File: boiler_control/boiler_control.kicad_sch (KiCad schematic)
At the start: 21 parts, among them J1 Conn_01x01, J3V3 Conn_01x03, J5V1 Conn_01x03, U2 MOUDLE-SEEEDUINO-XIAO-ESP32C3

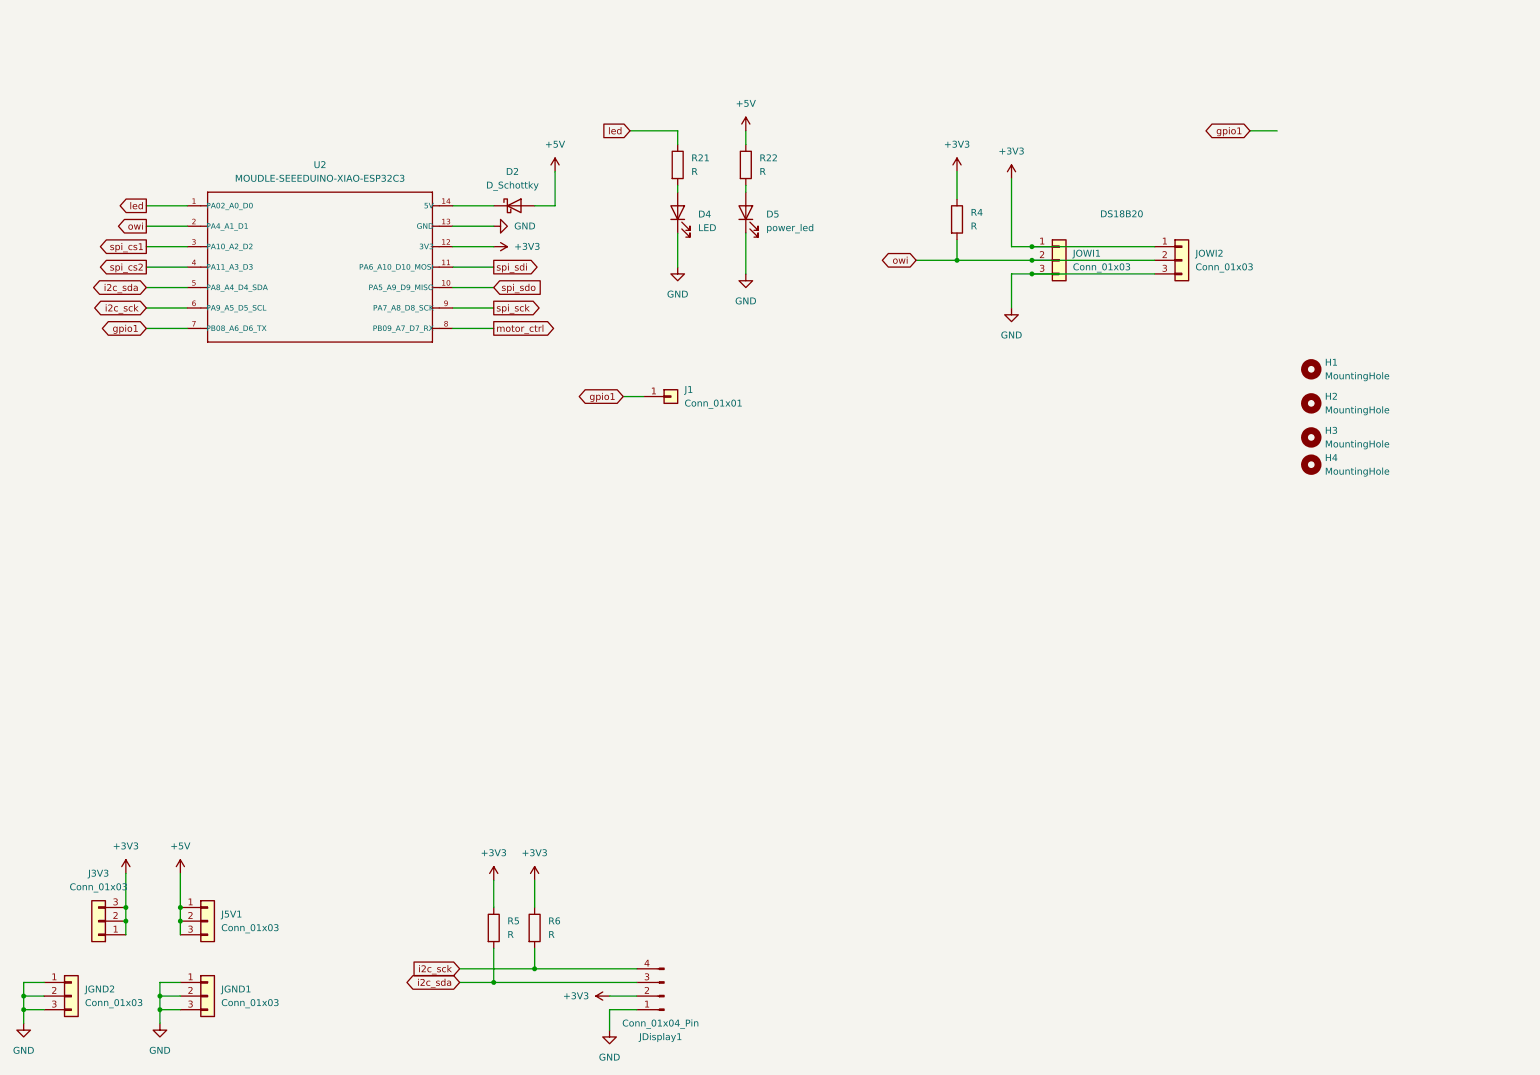
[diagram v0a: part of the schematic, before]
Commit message: Updating to v1.4 - pushed to order
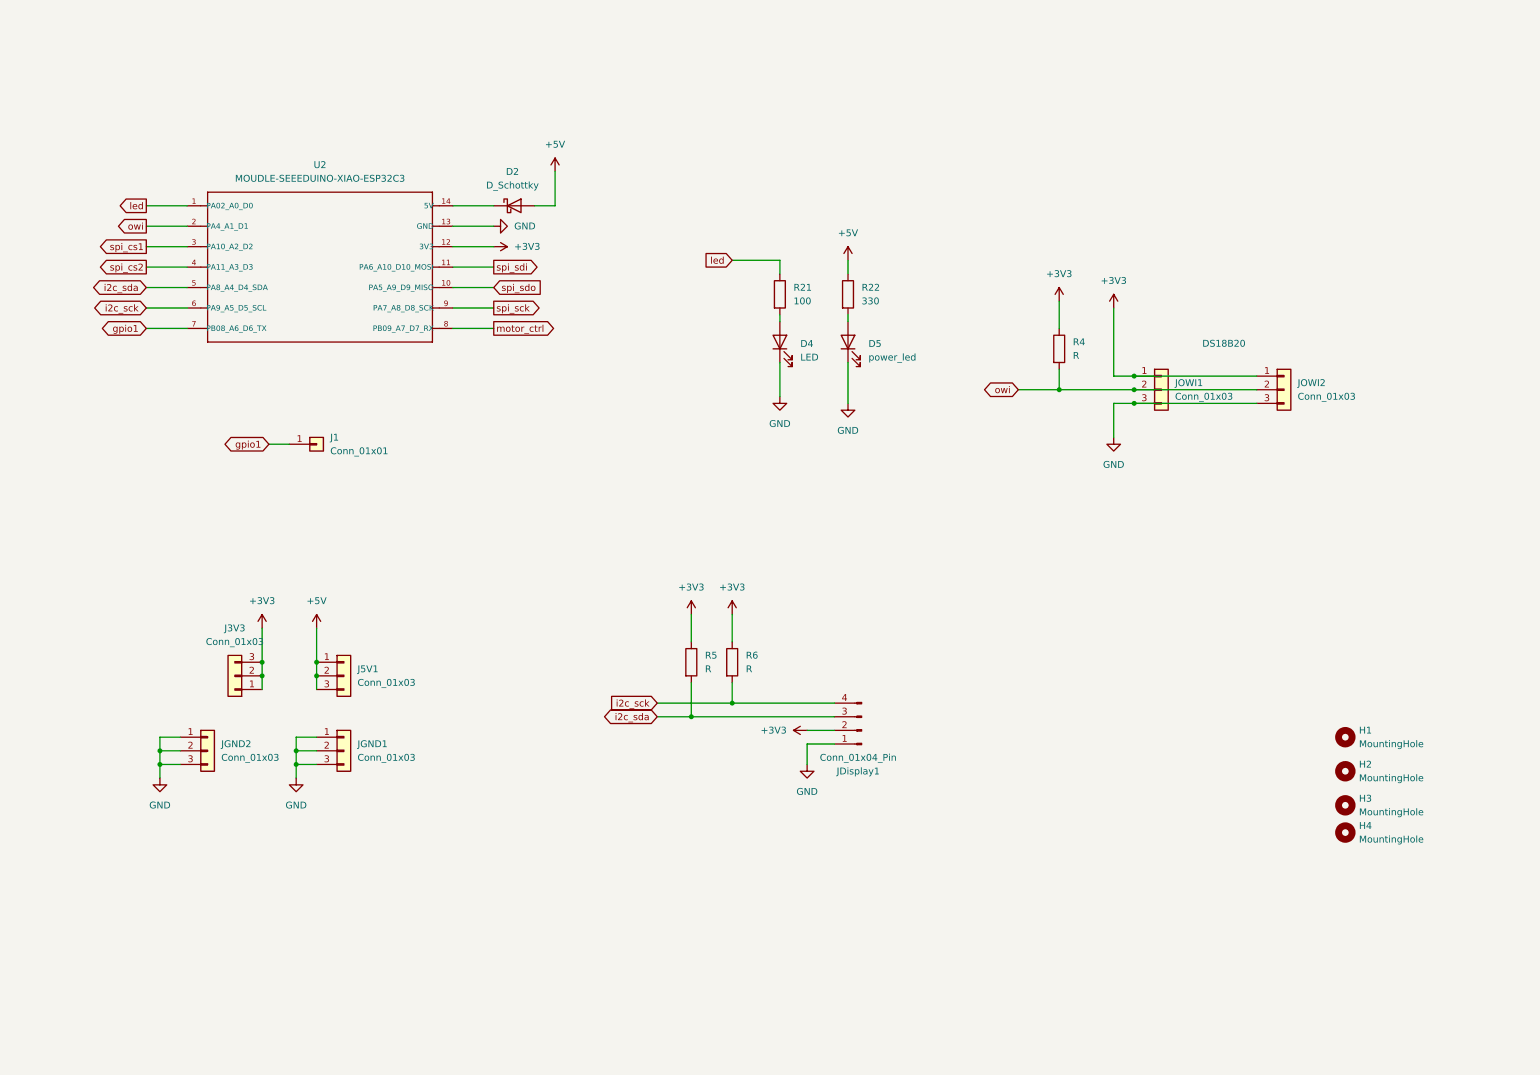
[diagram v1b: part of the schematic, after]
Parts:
- J1: footprint Connector_PinHeader_1.00mm:PinHeader_1x01_P1.00mm_Vertical -> Connector_PinHeader_2.54mm:PinHeader_1x01_P2.54mm_Vertical
- R21: value R -> 100
- R22: value R -> 330
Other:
- moved on the sheet: D4, D5, H1, H2, H3, H4, J1, J3V3, J5V1, JDisplay1, JGND1, JGND2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
